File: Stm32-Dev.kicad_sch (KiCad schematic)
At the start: 25 parts, among them J2 STDC14, U1 STM32F405RGTx, X1 25MHz

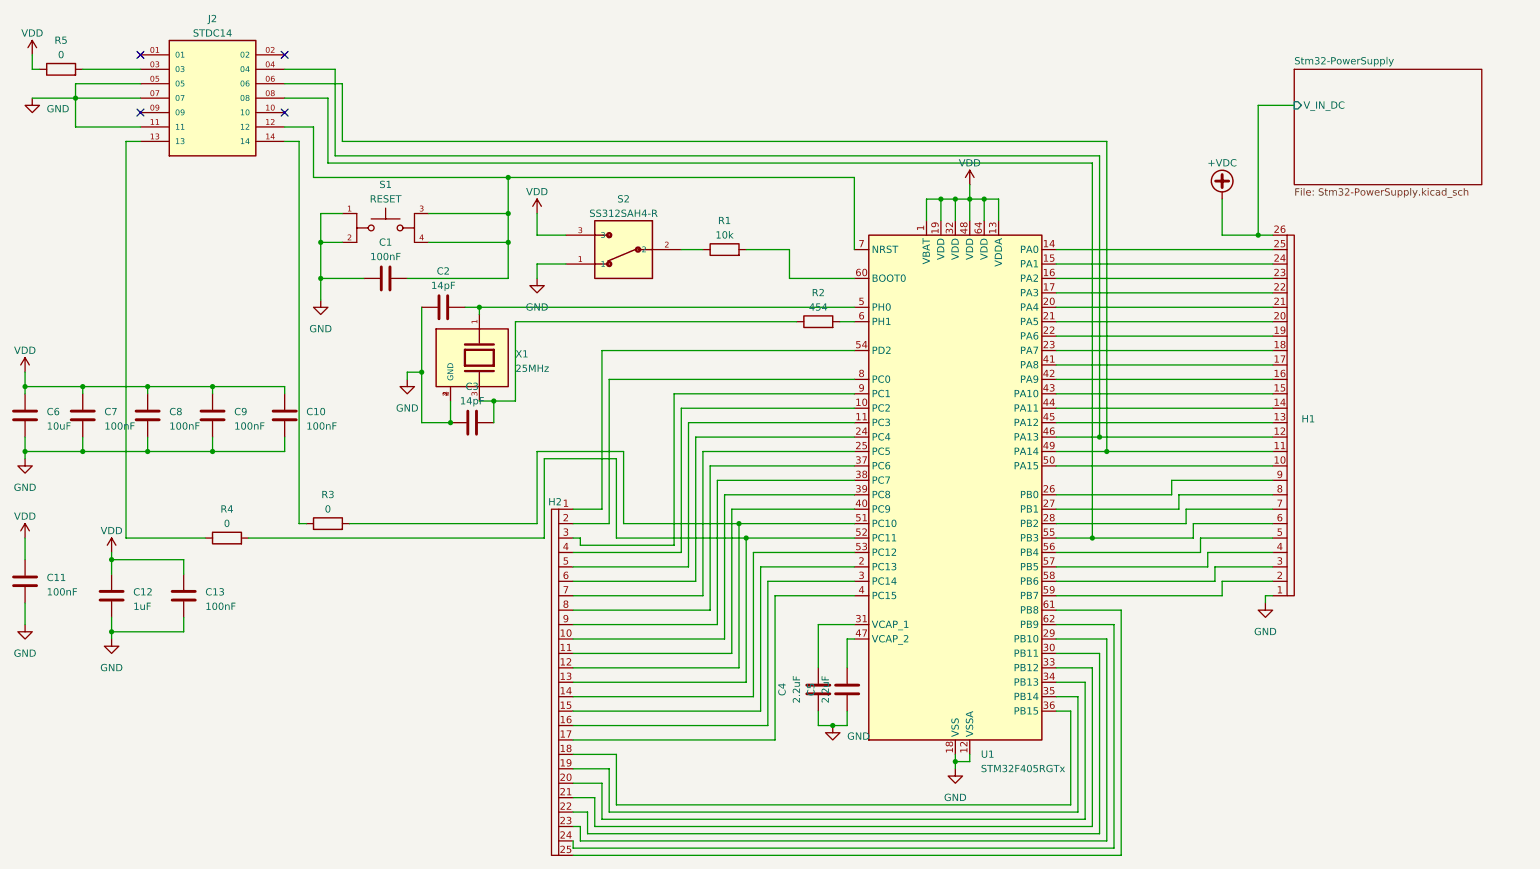
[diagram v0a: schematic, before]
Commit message: First Test Board
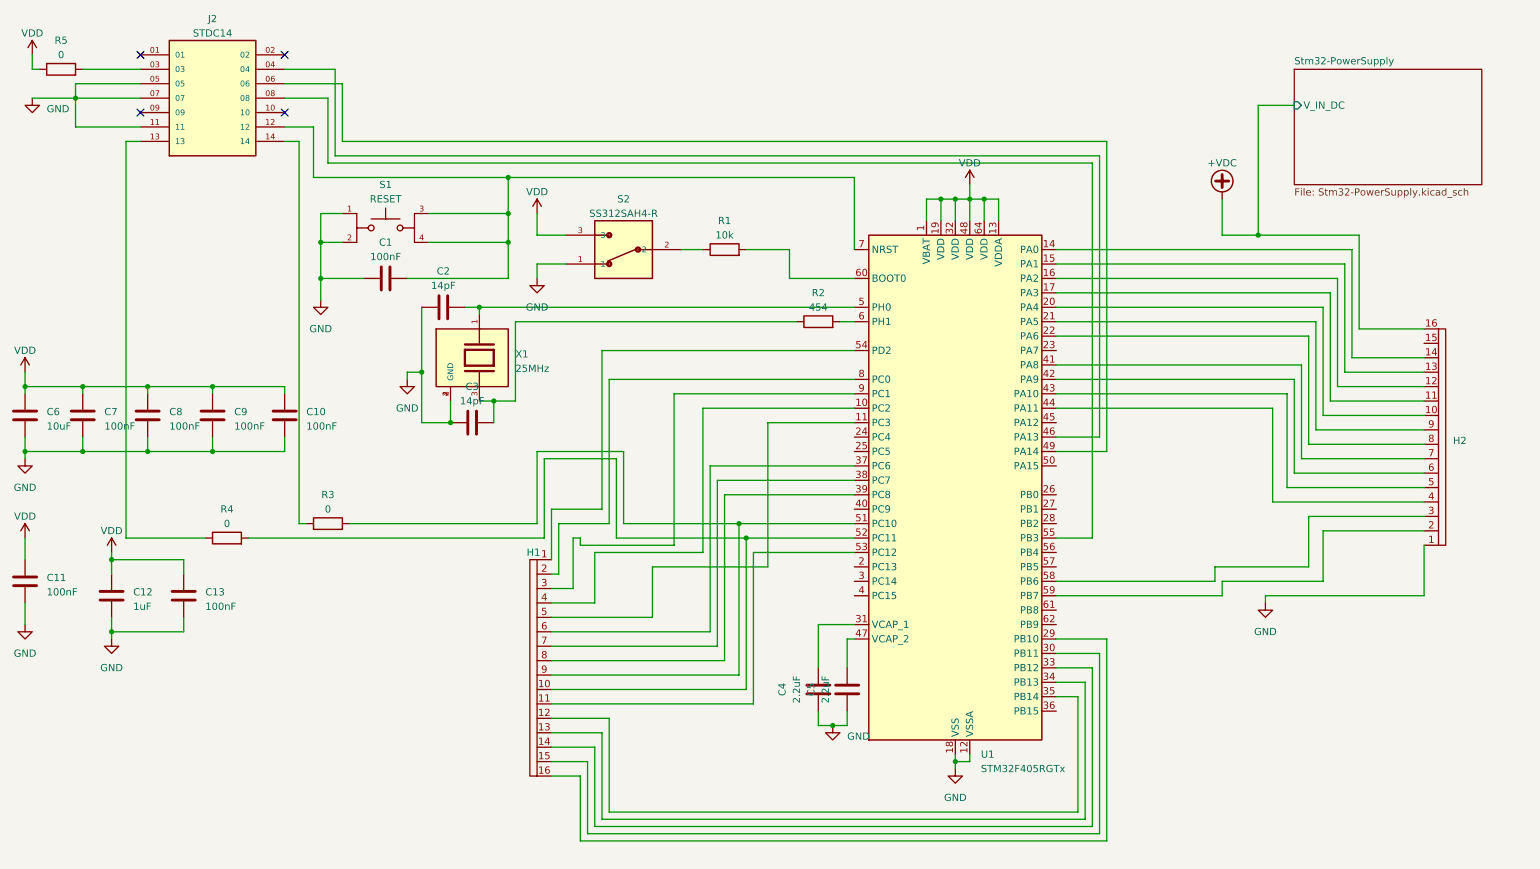
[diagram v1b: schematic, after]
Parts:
- removed H1: ~, 24_PIN_HEADER:HDRV26, symbol 24_PIN_HEADER:26_Header
- removed H2: ~, 24_PIN_HEADER:HDRV25, symbol 24_PIN_HEADER:25_Header
- added H1, H2: ~, 24_PIN_HEADER:HDRV16, symbol 24_PIN_HEADER:16_Header
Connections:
- net +VDC: now also H2.16
- net GND: now also H2.1
- net at U1.10 (PC2): now also H1.4
- net at U1.11 (PC3): now also H1.5
- net at U1.14 (PA0): now also H2.14
- net at U1.15 (PA1): now also H2.13
- net at U1.16 (PA2): now also H2.12
- net at U1.17 (PA3): now also H2.11
- net at U1.20 (PA4): now also H2.10
- net at U1.21 (PA5): now also H2.9
- net at U1.22 (PA6): now also H2.8
- net at U1.29 (PB10): now also H1.16
- net at U1.30 (PB11): now also H1.15
- net at U1.33 (PB12): now also H1.14
- net at U1.34 (PB13): now also H1.13
- net at U1.35 (PB14): now also H1.12
- net at U1.37 (PC6): now also H1.6
- net at U1.38 (PC7): now also H1.7
- net at U1.39 (PC8): now also H1.8
- net at U1.41 (PA8): now also H2.7
- net at U1.42 (PA9): now also H2.6
- net at U1.43 (PA10): now also H2.5
- net at U1.44 (PA11): now also H2.4
- net at R3.2, U1.51 (PC10): now also H1.9
- net at R4.2, U1.52 (PC11): now also H1.10
- net at U1.53 (PC12): now also H1.11
- net at U1.54 (PD2): now also H1.1
- net at U1.58 (PB6): now also H2.3
- net at U1.59 (PB7): now also H2.2
- net at U1.8 (PC0): now also H1.2
- net at U1.9 (PC1): now also H1.3
